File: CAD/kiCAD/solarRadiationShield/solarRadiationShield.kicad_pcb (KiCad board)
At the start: 2 copper layers, 13 x 37 mm, 4 parts

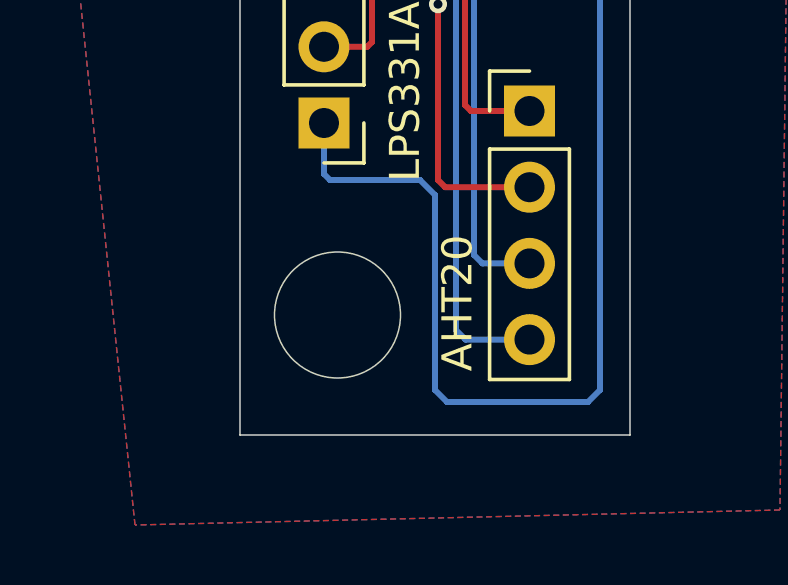
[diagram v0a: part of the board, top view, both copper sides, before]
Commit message: updates
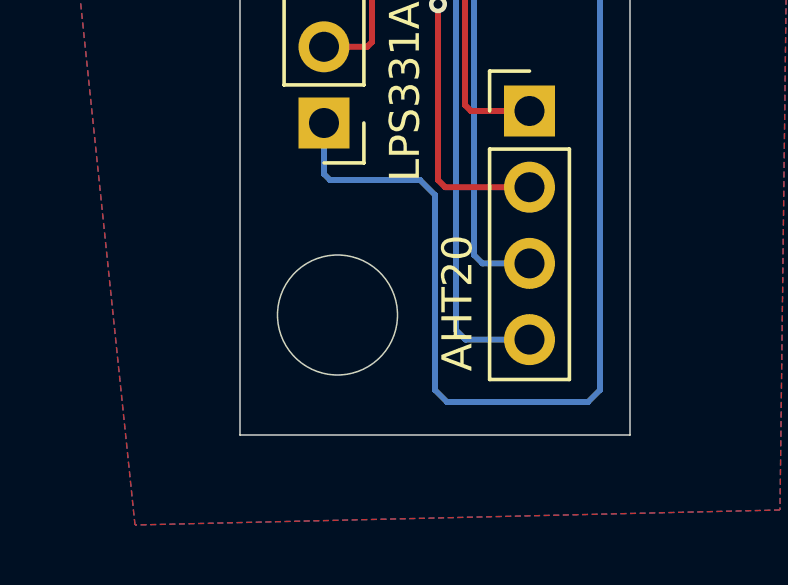
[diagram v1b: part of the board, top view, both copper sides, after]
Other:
- outline, holes or cut-outs redrawn
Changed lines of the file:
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@@
 	(gr_circle
 		(center 127.05 108.475)
-		(end 129.15 108.475)
+		(end 129.05 108.475)
 		(stroke
 			(width 0.05)
